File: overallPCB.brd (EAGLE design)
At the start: 160 x 100 mm, 40 parts, among them IC1 DS3231/SO, IC4 CP2104, Q7 mmbt2222, Q8 mmbt2222, Q9 DMG3415U, SW3 KMR2, U2 TB6612 SSOP, U5 MCP73831T-2ACI/OT, U6 AP2112-3.3, X7 ESP32_WROOM32_SKINNY, X8 20329, X9 JSTPH

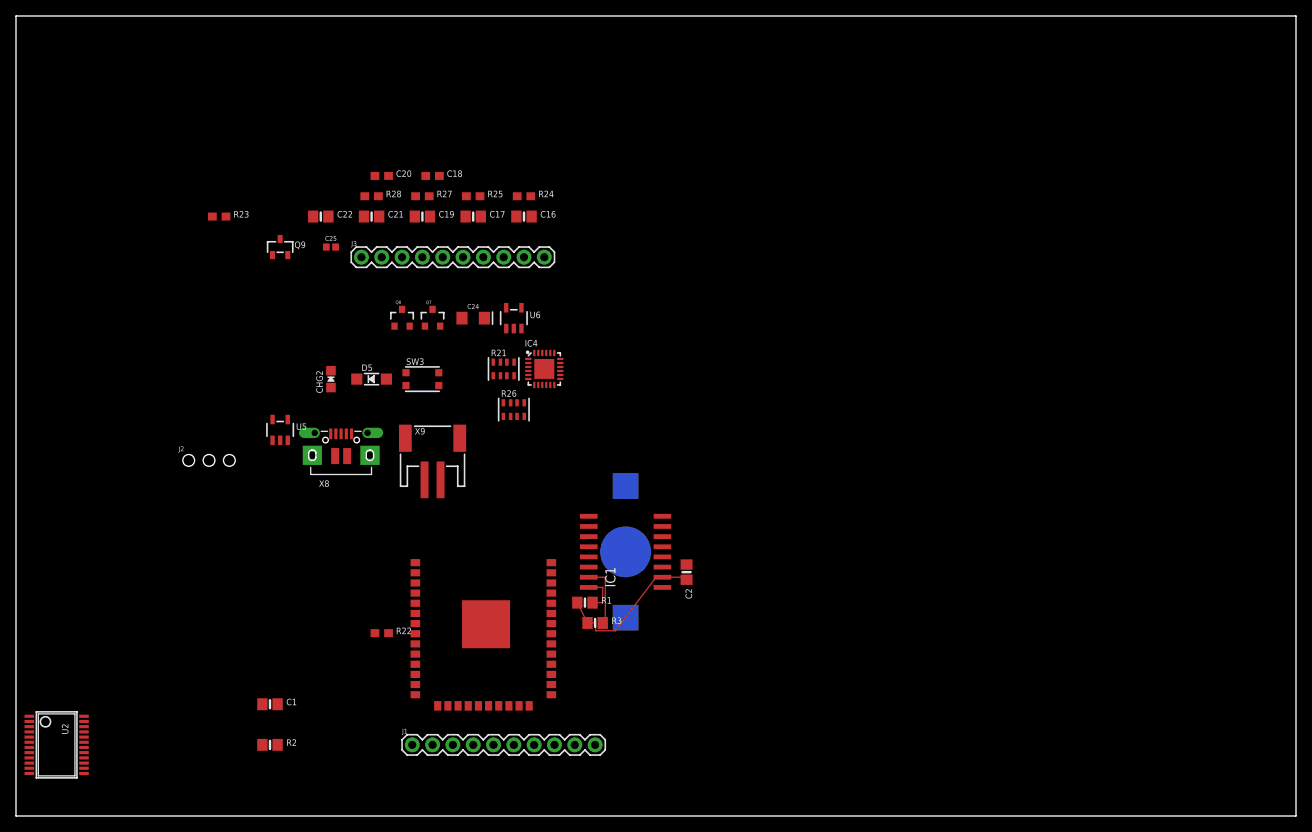
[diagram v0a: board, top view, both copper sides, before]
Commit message: Add files via upload
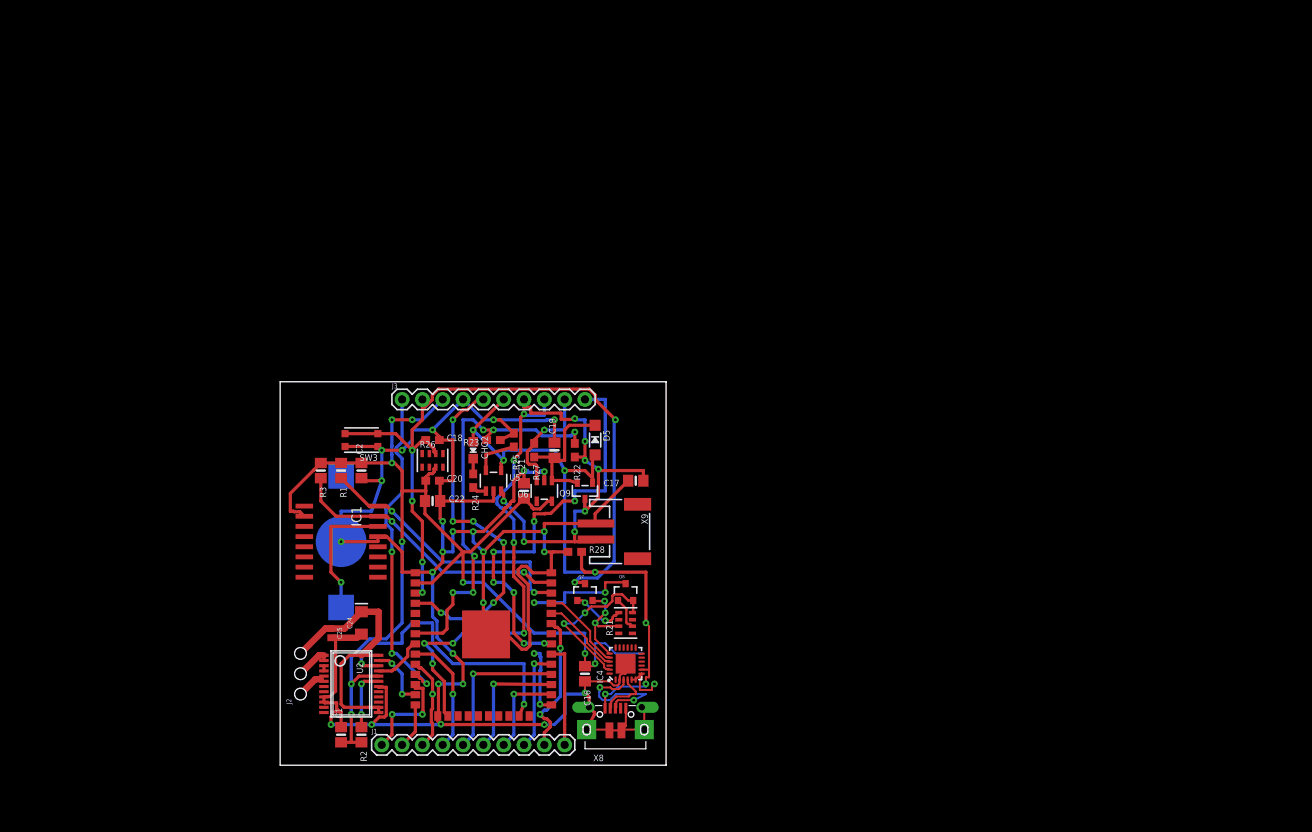
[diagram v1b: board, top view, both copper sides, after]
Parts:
- moved C16 57.7 mm to (71.1, 17.8), turned to 270 degrees
- moved R28 51.2 mm to (69.8, 33.0)
- moved Q9 48.8 mm to (71.1, 40.6), turned to 180 degrees
- moved X8 48.5 mm to (74.9, 12.7)
- moved C25 48.3 mm to (39.4, 22.9), turned to 270 degrees
- moved R23 44.2 mm to (59.7, 47.0), turned to 180 degrees
- moved Q8 44.2 mm to (76.2, 27.9)
- moved C2 42.6 mm to (43.2, 43.2), turned to 90 degrees
- moved C24 40.6 mm to (43.2, 24.1), turned to 90 degrees
- moved C21 39.2 mm to (63.5, 40.6), turned to 90 degrees
- moved R3 39.2 mm to (38.1, 43.2), turned to 270 degrees
- moved Q7 39.2 mm to (71.1, 27.9)
- moved C17 38.8 mm to (77.5, 41.9), turned to 180 degrees
- moved C20 38.6 mm to (52.1, 41.9)
- moved C22 38.2 mm to (52.1, 39.4)
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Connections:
- net 3.3V: now also J3.3; no longer J3.1
- net A0_DAC2: now also J3.1; no longer J3.6
- net CONTROL_BUTTON: now also J1.7; no longer J1.2
- net EN: now also J3.9; no longer J3.10
- net FINGERPRINT_RX: now also J1.5; no longer J1.7
- net FINGERPRINT_TX: now also J1.6; no longer J1.8
- net GND: now also J3.4; no longer J3.2
- net GPIO19: now also J3.10; no longer J3.3
- net IO13_A12: now also J3.8; no longer J3.4
- net MOTOR_C1: now also J1.1; no longer J1.9
- net MOTOR_C2: now also J1.4; no longer J1.10
- net OLED_CS: now also J1.9; no longer J1.6
- net OLED_DC: now also J1.3; no longer J1.5
- net OLED_MOSI: now also J1.10; no longer J1.4
- net OLED_SCK: now also J1.8; no longer J1.3
- net RESET: now also J3.2; no longer J3.9
- net SCANNER_BUTTON: now also J1.2; no longer J1.1
- net VBUS: now also J3.6; no longer J3.8
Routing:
- net GND: track 0.00 -> 309.2 mm, vias 0 -> 26
- net 3.3V: track 20.3 -> 159.0 mm, vias 0 -> 10
- net RESET: track 0.00 -> 92.3 mm, vias 0 -> 6
- net VBUS: track 0.00 -> 81.5 mm, vias 0 -> 7
- net IO13_A12: track 0.00 -> 58.3 mm, vias 0 -> 7
- net VBAT: track 0.00 -> 57.0 mm, vias 0 -> 8
- net A13_I35: track 0.00 -> 52.3 mm, vias 0 -> 6
- net GPIO19: track 0.00 -> 51.9 mm, vias 0 -> 7
- net A4_IO36: track 0.00 -> 44.2 mm, vias 0 -> 6
- net A0_DAC2: track 0.00 -> 41.4 mm, vias 0 -> 3
- net AIN2: track 0.00 -> 36.6 mm, vias 0 -> 2
- net VM+: track 0.00 -> 34.0 mm
- net SCL: track 4.60 -> 34.6 mm, vias 0 -> 2
- net SDA: track 7.78 -> 36.7 mm, vias 0 -> 2
- net GPIO0: track 0.00 -> 22.9 mm, vias 0 -> 4
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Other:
- board size 160 x 100 mm -> 48.2 x 47.9 mm
